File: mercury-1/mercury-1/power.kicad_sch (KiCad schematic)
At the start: 29 parts, among them P1 Logic Kill Switch, U1 XT60PW-F, U2 TPS1HA08AQPWPRQ1, U3 LT8612EUDE#PBF

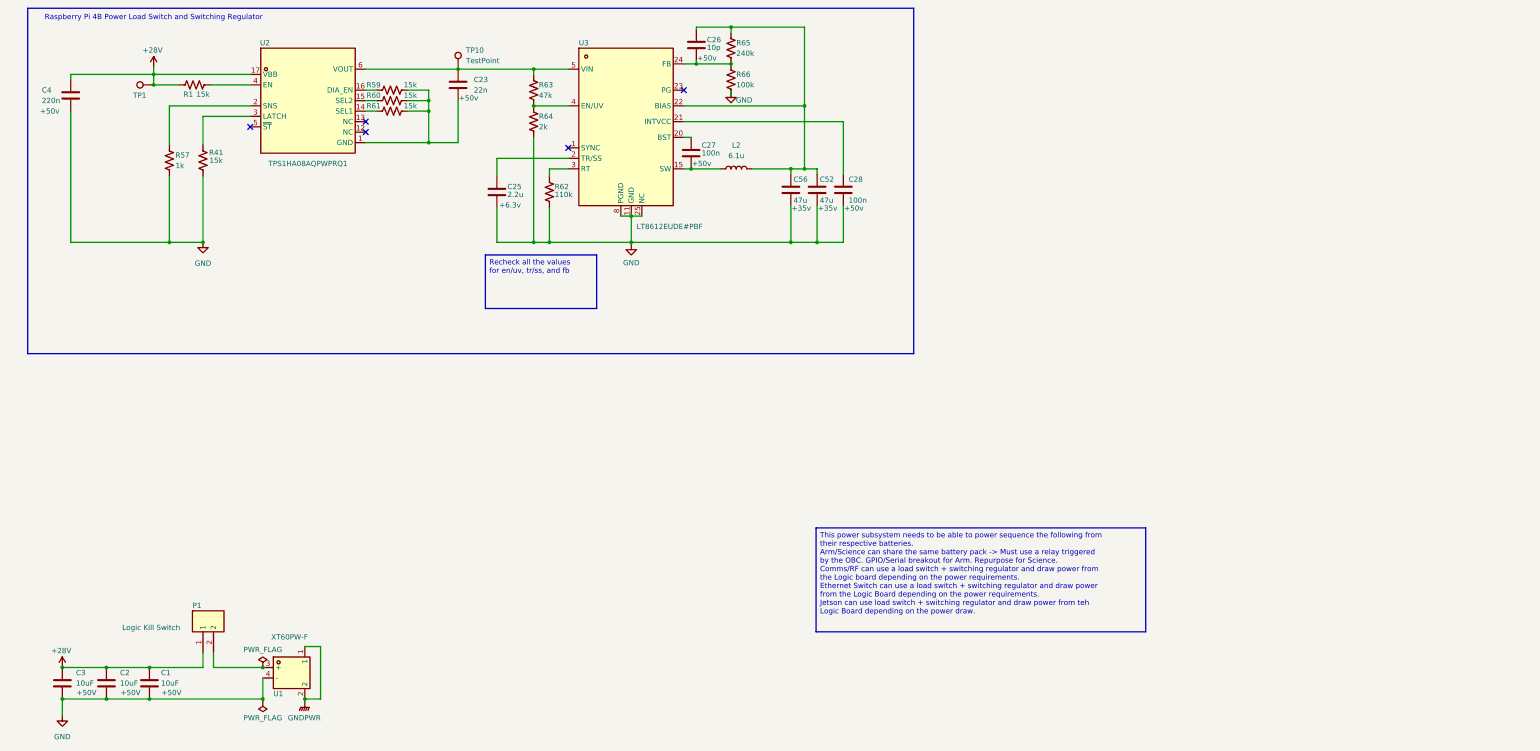
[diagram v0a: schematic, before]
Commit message: Draw.io updated
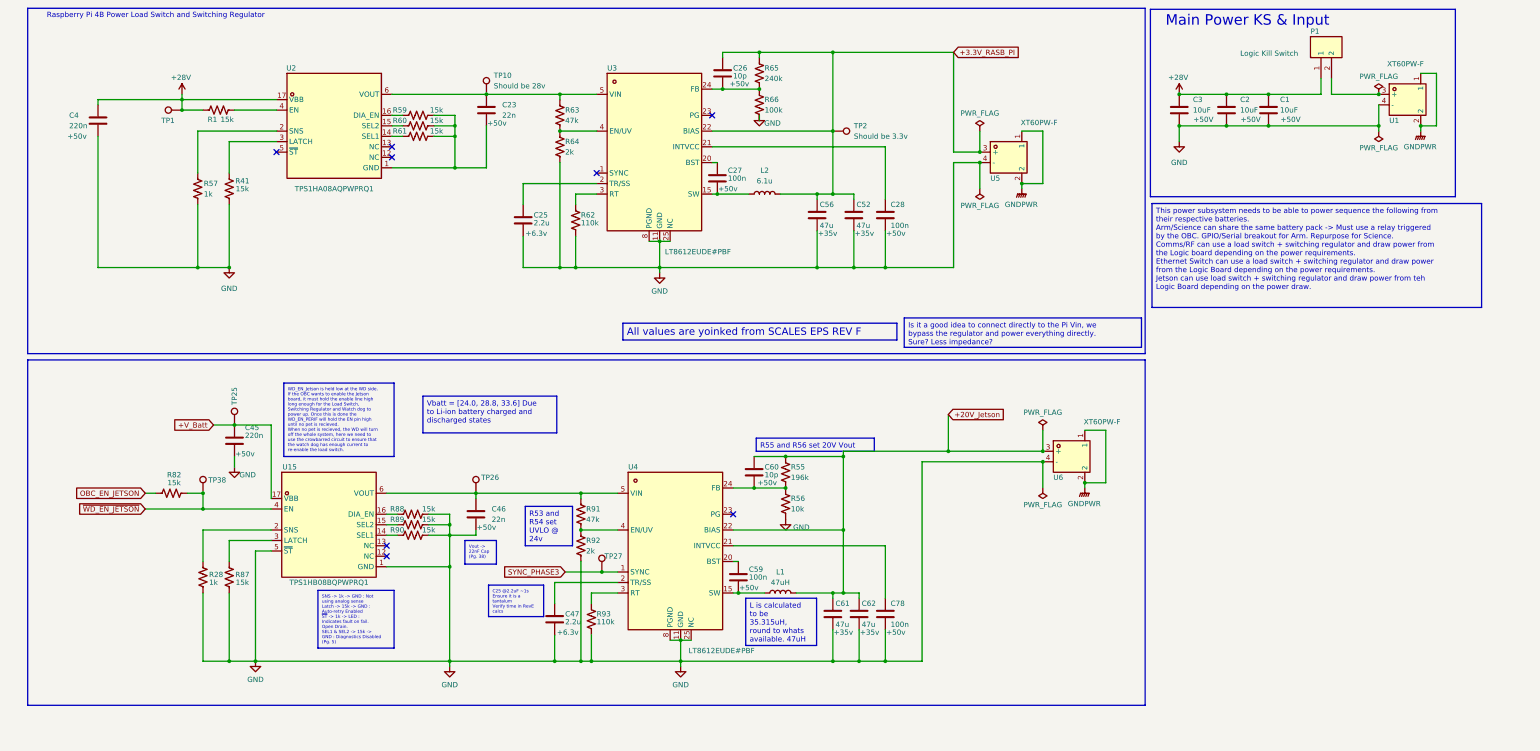
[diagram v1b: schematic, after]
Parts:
- added C45: 220n, EPS:C0402, symbol Device:C
- added C46: 22n, EPS:C0402, symbol Device:C
- added C47: 2.2u, EPS:C0402, symbol Device:C
- added C59, C78: 100n, EPS:C0402, symbol Device:C
- added C60: 10p, EPS:C0402, symbol Device:C
- added C61, C62: 47u, EPS:CAP-SMD_L7.3-W4.3-FD, symbol Device:C
- added L1: 47uH, EPS:IND-SMD_L10.7-W10.0_ETQP5MXXXX, symbol Device:L
- added R28: 1k, EPS:R0402, symbol Device:R_US
- added R55: 196k, EPS:R0402, symbol Device:R_US
- added R56: 10k, EPS:R0402, symbol Device:R_US
- added R82, R87, R88, R89, R90: 15k, EPS:R0402, symbol Device:R_US
- added R91: 47k, EPS:R0402, symbol Device:R_US
- added R92: 2k, EPS:R0402, symbol Device:R_US
- added R93: 110k, EPS:R0402, symbol Device:R_US
- added TP2: Should be 3.3v, TestPoint:TestPoint_Pad_1.0x1.0mm, symbol EPS:TestPoint
- added TP25, TP26, TP27, TP38: TestPoint, TestPoint:TestPoint_Pad_1.0x1.0mm, symbol EPS:TestPoint
- added U15: TPS1HB08BQPWPRQ1, EPS:HTSSOP-16_L5.0-W4.4-P0.65-LS6.4-TL-EP2.9, symbol EPS:TPS1HB08BQPWPRQ1
- added U4: LT8612EUDE#PBF, EPS:QFN-28_L6.0-W3.0-P0.50-BL-EP, symbol EPS:LT8612EUDE#PBF
- added U5, U6: XT60PW-F, logic_board:TH_2P-XT60PW-F, symbol logic_board:XT60PW-F_C428722
- TP10: value TestPoint -> Should be 28v
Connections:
- net GND: now also C45.2, C46.2, C47.2, C61.2, C62.2, C78.2, R28.1, R56.2, R87.2, R88.2, R89.2, R90.2, R92.2, R93.2, U15.1 (GND), U15.5 (~{ST}), U4.11 (GND), U4.25 (NC), U4.8 (PGND), U5.4 (-), U6.4 (-)
- net GNDPWR: now also U5.1, U5.2, U6.1, U6.2
- net +3.3V_RASB_PI: now reaches C26.1, C52.1, C56.1, L2.2, R65.1, U3.22 (BIAS)
- net +3.3V_RASB_PI: now also TP2.1, U5.3 (+)
- new net: R89.1, U15.15 (SEL2)
- new net: C46.1, R91.1, TP26.1, U15.6 (VOUT), U4.5 (VIN)
- new net: R91.2, R92.1, U4.4 (EN/UV)
- new net: C60.2, R55.2, R56.1, U4.24 (FB)
- new net: R90.1, U15.14 (SEL1)
- new net: C78.1, U4.21 (INTVCC)
- new net: C59.2, L1.1, U4.15 (SW)
- new net: R88.1, U15.16 (DIA_EN)
- new net: R28.2, U15.2 (SNS)
- new net: C47.1, U4.2 (TR/SS)
- new net: C59.1, U4.20 (BST)
- new net: R93.1, U4.3 (RT)
- new net: R87.1, U15.3 (LATCH)
- new net +20V_Jetson: C60.1, C61.1, C62.1, L1.2, R55.1, U4.22 (BIAS), U6.3 (+)
- new net +V_Batt: C45.1, TP25.1, U15.17 (VBB)
- new net OBC_EN_JETSON: R82.2
- new net SYNC_PHASE3: TP27.1, U4.1 (SYNC)
- new net ~{WD_EN_JETSON}: R82.1, TP38.1, U15.4 (EN)
- no-connect marks 5 -> 8
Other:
- note added: "Main Power KS & Input"
- moved on the sheet: C1, C2, C23, C25, C26, C27, C28, C3, C4, C52, C56, L2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
